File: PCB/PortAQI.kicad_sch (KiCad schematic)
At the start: 3 parts, among them J1 OLED Display, U1 ESP32-WROOM-32, U2 DIP-GAS-MQ-2_6P-D19MM_

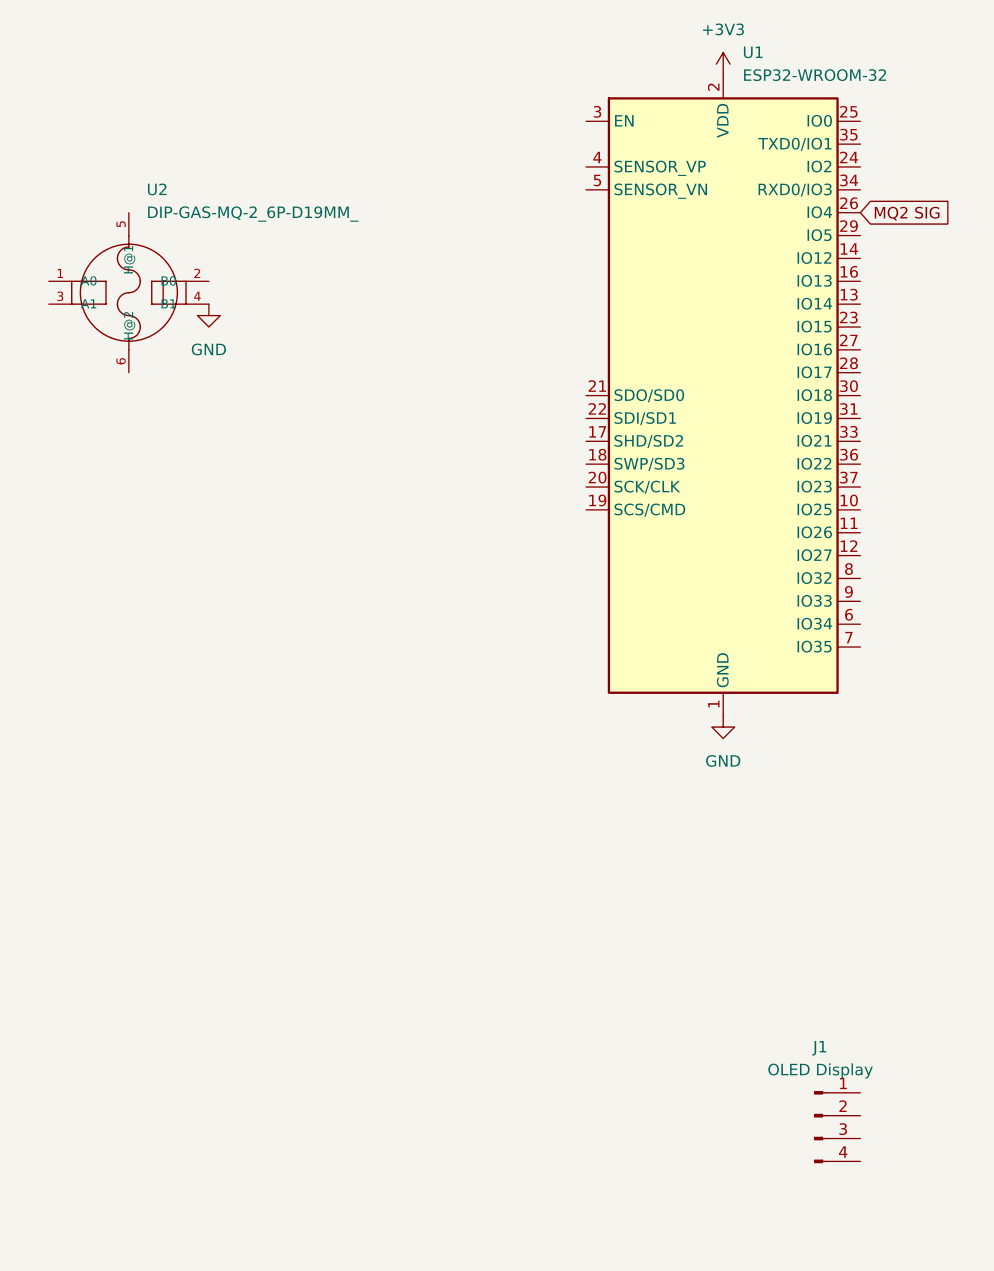
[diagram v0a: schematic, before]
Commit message: First draft of Schematic
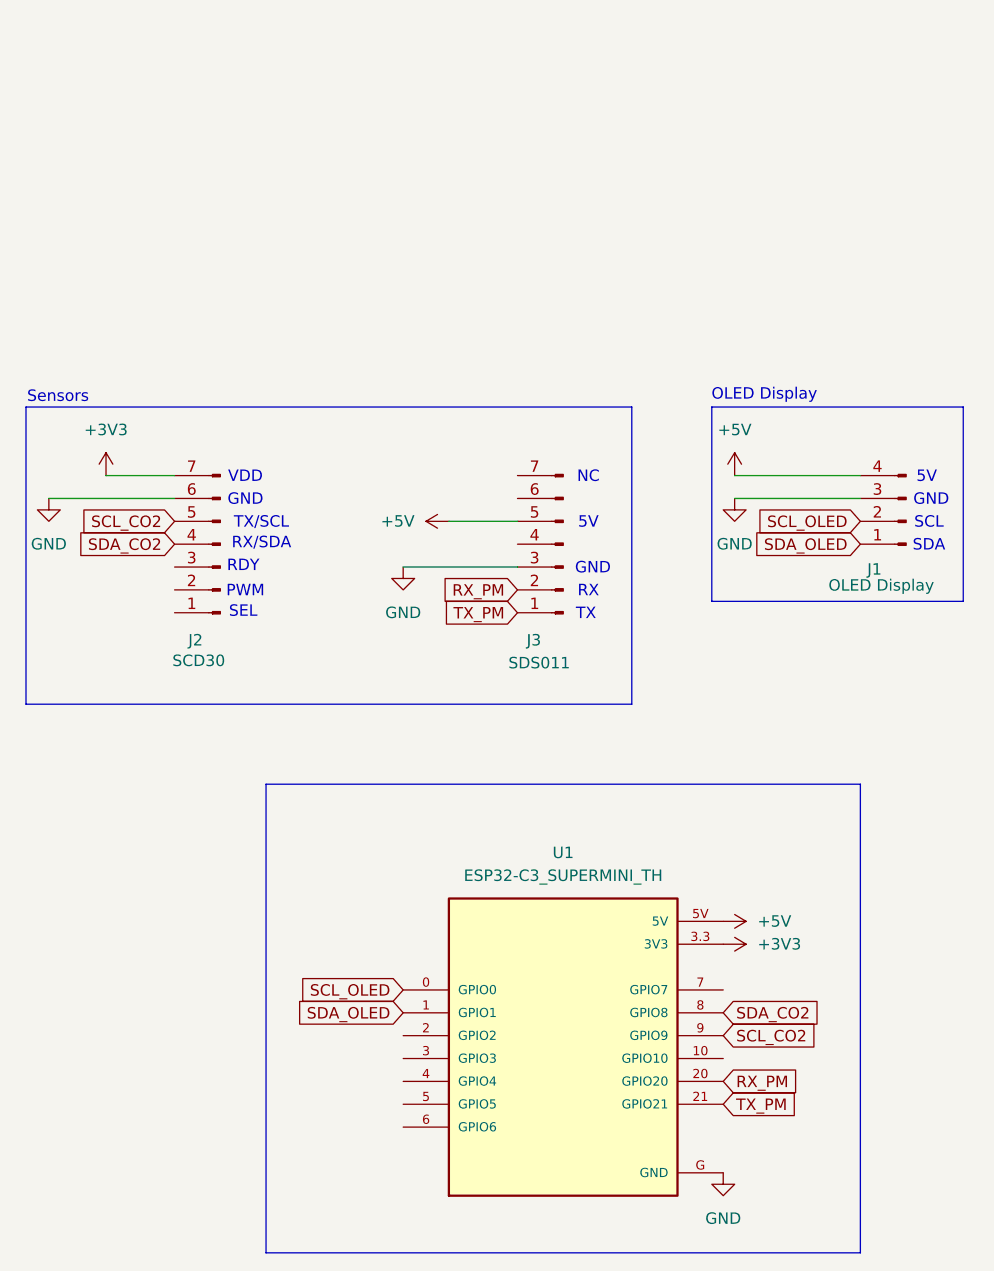
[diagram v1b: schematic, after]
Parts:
- removed U1: ESP32-WROOM-32, RF_Module:ESP32-WROOM-32, symbol RF_Module:ESP32-WROOM-32
- removed U2: DIP-GAS-MQ-2_6P-D19MM_, DIP-GAS-MQ-2_6P-D19MM_:SNR6-D19.0MM, symbol DIP-GAS-MQ-2_6P-D19MM_:DIP-GAS-MQ-2_6P-D19MM_
- added J2: SCD30, symbol Connector:Conn_01x07_Pin
- added J3: SDS011, symbol Connector:Conn_01x07_Pin
- added U1: ESP32-C3_SUPERMINI_TH, ESP32-C3_SUPERMINI_TH:MODULE_ESP32-C3_SUPERMINI_TH, symbol ESP32-C3_SUPERMINI_TH:ESP32-C3_SUPERMINI_TH
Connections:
- net +3V3: now also J2.7 (Pin_7), U1.3.3 (3V3)
- net GND: now also J1.3 (Pin_3), J2.6 (Pin_6), J3.3 (Pin_3), U1.G (GND)
- net SDA_OLED: now reaches J1.1 (Pin_1)
- net SDA_OLED: now also U1.1 (GPIO1)
- net SCL_OLED: now reaches J1.2 (Pin_2)
- net SCL_OLED: now also U1.0 (GPIO0)
- net +5V: now reaches J1.4 (Pin_4)
- net +5V: now also J3.5 (Pin_5), U1.5V
- new net RX_PM: J3.2 (Pin_2), U1.20 (GPIO20)
- new net SCL_CO2: J2.5 (Pin_5), U1.9 (GPIO9)
- new net SDA_CO2: J2.4 (Pin_4), U1.8 (GPIO8)
- new net TX_PM: J3.1 (Pin_1), U1.21 (GPIO21)
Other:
- note added: "5V"
- note added: "GND"
- note added: "NC"
- note added: "OLED Display"
- note added: "PWM"
- note added: "RDY"
- note added: "RX"
- note added: "RX/SDA"
- note added: "SCL"
- note added: "SDA"
- note added: "SEL"
- note added: "Sensors"
- note added: "TX"
- note added: "TX/SCL"
- note added: "VDD"
- moved on the sheet: J1

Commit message: Added sensor functionality
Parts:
- J1: footprint footprints:SSD1306-0.91-OLED-4pin-128x32 -> (none)
- U1: footprint ESP32-C3_SUPERMINI_TH:MODULE_ESP32-C3_SUPERMINI_TH -> footprints:MODULE_ESP32-C3_SUPERMINI_TH
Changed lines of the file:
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@@
 			)
 		)
-		(property "Footprint" "footprints:SSD1306-0.91-OLED-4pin-128x32"
+		(property "Footprint" ""
 			(at 273.05 73.66 0)
 			(effects
@@
 			)
 		)
-		(property "Footprint" "ESP32-C3_SUPERMINI_TH:MODULE_ESP32-C3_SUPERMINI_TH"
+		(property "Footprint" "footprints:MODULE_ESP32-C3_SUPERMINI_TH"
 			(at 234.95 130.81 0)
 			(effects
